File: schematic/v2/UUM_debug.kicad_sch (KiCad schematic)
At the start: 16 parts, among them J16 DSM_DBG, J20 USB_A, U33 CH340G, Y2 Crystal

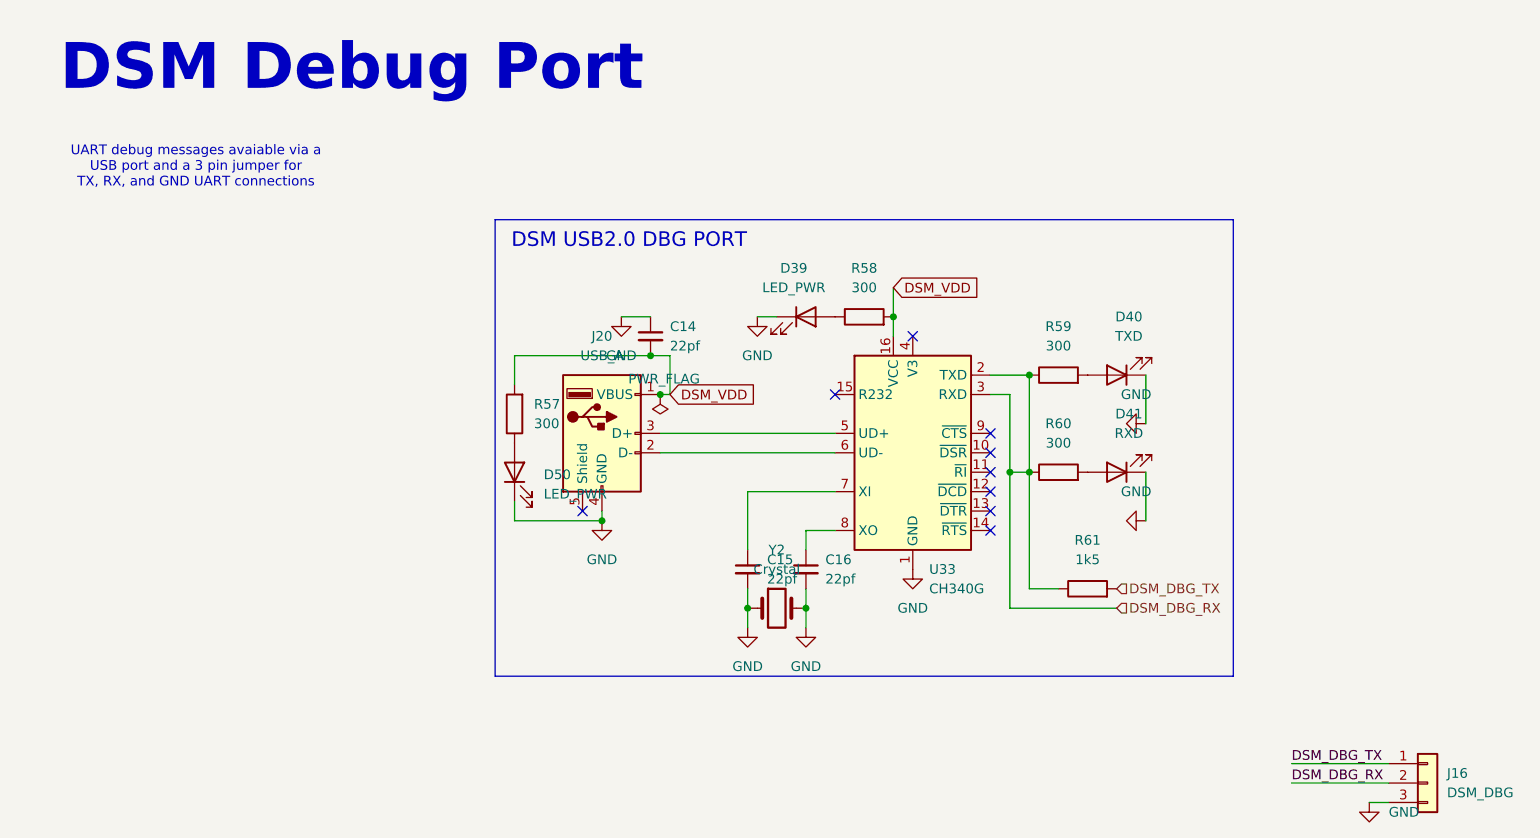
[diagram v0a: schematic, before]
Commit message: no errors in the ERC!
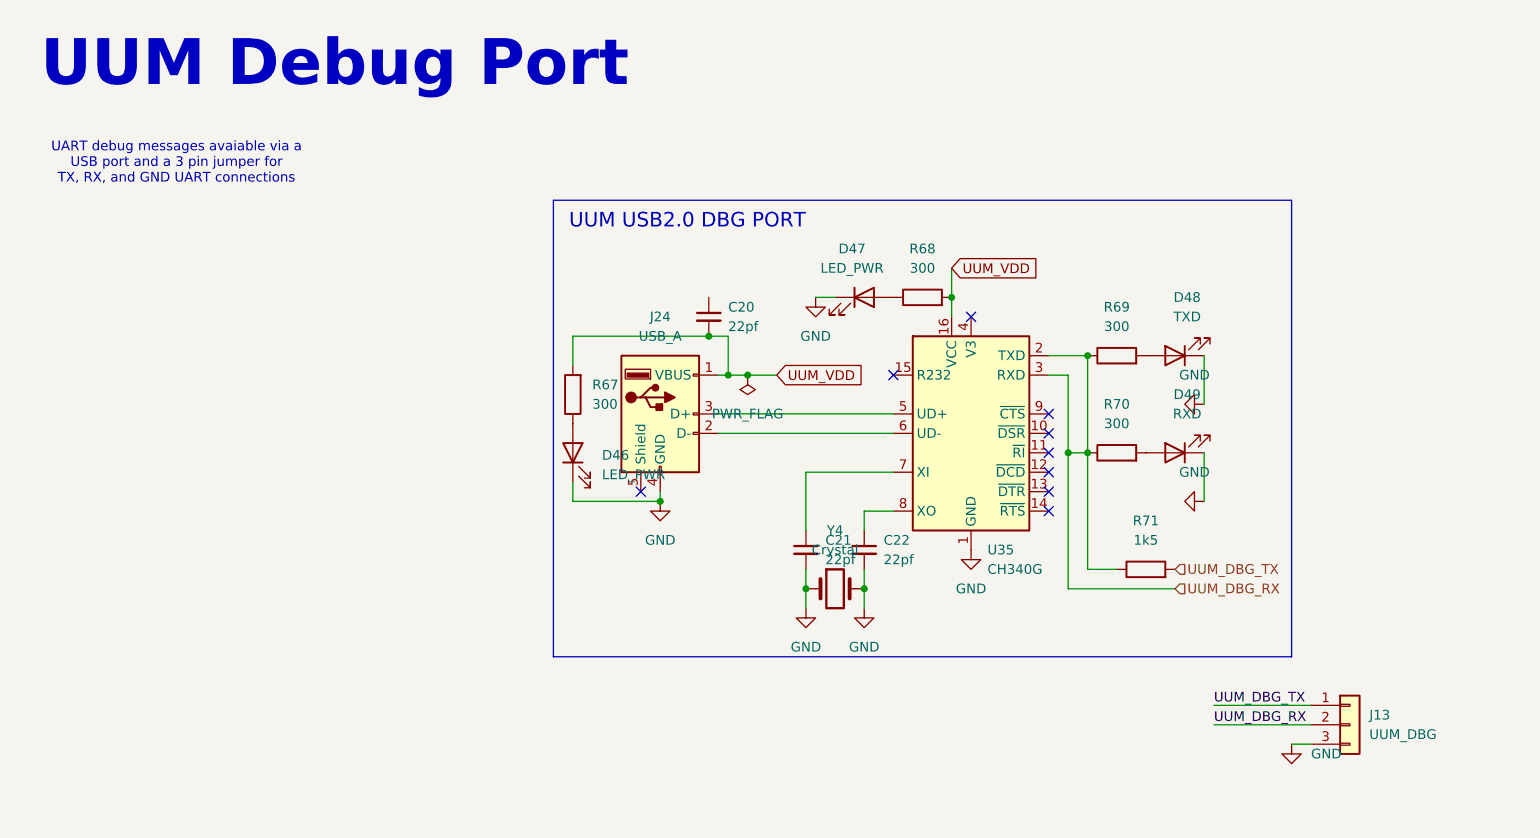
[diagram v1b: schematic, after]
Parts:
- removed C14, C15, C16: 22pf, Capacitor_SMD:C_0805_2012Metric, symbol Device:C_Small
- removed D39, D50: LED_PWR, LED_SMD:LED_0603_1608Metric, symbol Device:LED
- removed D40: TXD, LED_SMD:LED_0603_1608Metric, symbol Device:LED
- removed D41: RXD, LED_SMD:LED_0603_1608Metric, symbol Device:LED
- removed J16: DSM_DBG, Connector_PinHeader_1.00mm:PinHeader_1x03_P1.00mm_Horizontal, symbol Connector_Generic:Conn_01x03
- removed J20: USB_A, Connector_USB:USB_A_CNCTech_1001-011-01101_Horizontal, symbol Connector:USB_A
- removed R57, R58, R59, R60: 300, Resistor_SMD:R_0805_2012Metric_Pad1.20x1.40mm_HandSolder, symbol Device:R
- removed R61: 1k5, Resistor_SMD:R_0805_2012Metric_Pad1.20x1.40mm_HandSolder, symbol Device:R
- removed U33: CH340G, Package_SO:SOIC-16_3.9x9.9mm_P1.27mm, symbol Interface_USB:CH340G
- removed Y2: Crystal, symbol Device:Crystal
- added C20, C21, C22: 22pf, Capacitor_SMD:C_0805_2012Metric, symbol Device:C_Small
- added D46, D47: LED_PWR, LED_SMD:LED_0603_1608Metric, symbol Device:LED
- added D48: TXD, LED_SMD:LED_0603_1608Metric, symbol Device:LED
- added D49: RXD, LED_SMD:LED_0603_1608Metric, symbol Device:LED
- added J13: UUM_DBG, Connector_PinHeader_1.00mm:PinHeader_1x03_P1.00mm_Horizontal, symbol Connector_Generic:Conn_01x03
- added J24: USB_A, Connector_USB:USB_A_CNCTech_1001-011-01101_Horizontal, symbol Connector:USB_A
- added R67, R68, R69, R70: 300, Resistor_SMD:R_0805_2012Metric_Pad1.20x1.40mm_HandSolder, symbol Device:R
- added R71: 1k5, Resistor_SMD:R_0805_2012Metric_Pad1.20x1.40mm_HandSolder, symbol Device:R
- added U35: CH340G, Package_SO:SOIC-16_3.9x9.9mm_P1.27mm, symbol Interface_USB:CH340G
- added Y4: Crystal, symbol Device:Crystal
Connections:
- net GND: now also C21.2, C22.2, D46.1 (K), D47.1 (K), D48.1 (K), D49.1 (K), J13.3 (Pin_3), J24.4 (GND), U35.1 (GND), Y4.1, Y4.2
- new net: C21.1, U35.7 (XI)
- new net: J24.2 (D-), U35.6 (UD-)
- new net: J24.3 (D+), U35.5 (UD+)
- new net: D49.2 (A), R70.2
- new net: D48.2 (A), R69.2
- new net: D47.2 (A), R68.1
- new net: C22.1, U35.8 (XO)
- new net: D46.2 (A), R67.1
- new net UUM_DBG_RX: J13.2 (Pin_2), R69.1, R70.1, R71.1, U35.2 (TXD), U35.3 (RXD)
- new net UUM_DBG_TX: J13.1 (Pin_1), R71.2
- new net UUM_VDD: C20.2, J24.1 (VBUS), R67.2, R68.2, U35.16 (VCC)
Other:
- note added: "UUM Debug Port"
- note added: "UUM USB2.0 DBG PORT"
- note removed: "DSM Debug Port"
- note removed: "DSM USB2.0 DBG PORT"
